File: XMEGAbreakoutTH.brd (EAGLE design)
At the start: 62.2 x 48.3 mm, 26 parts, among them IC1 XMEGA16A4

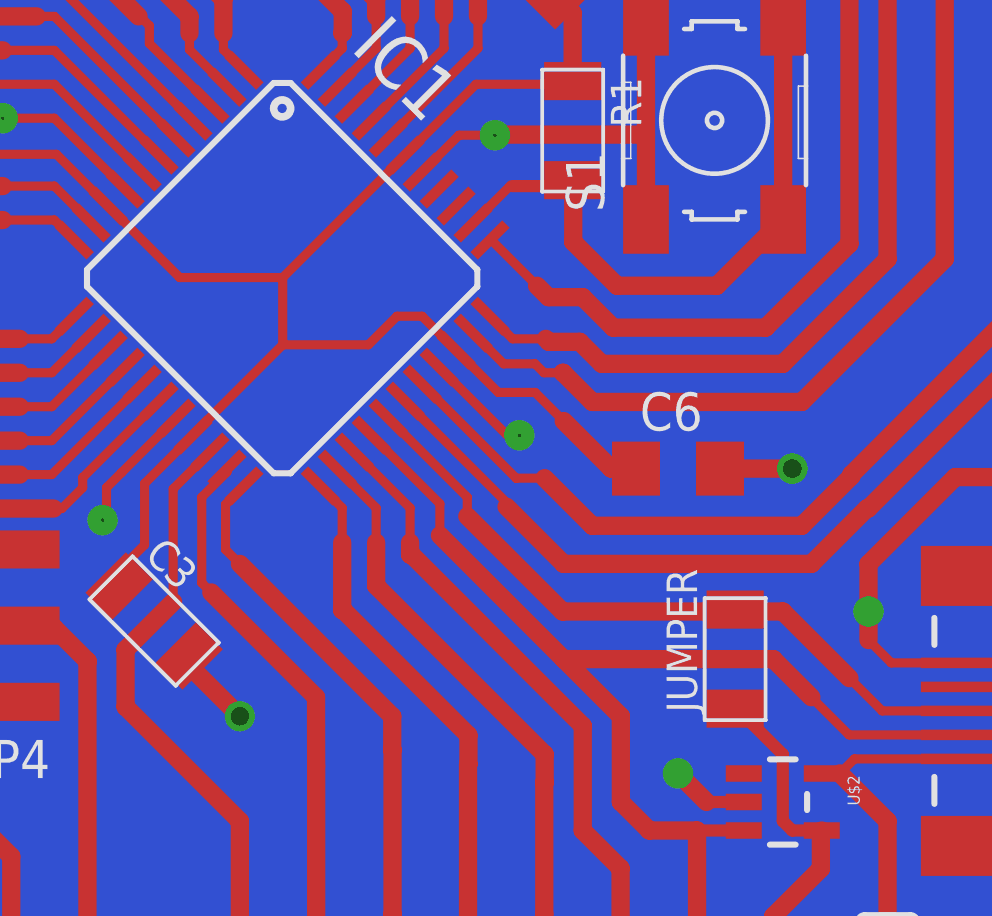
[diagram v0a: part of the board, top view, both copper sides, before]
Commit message: 600dpi
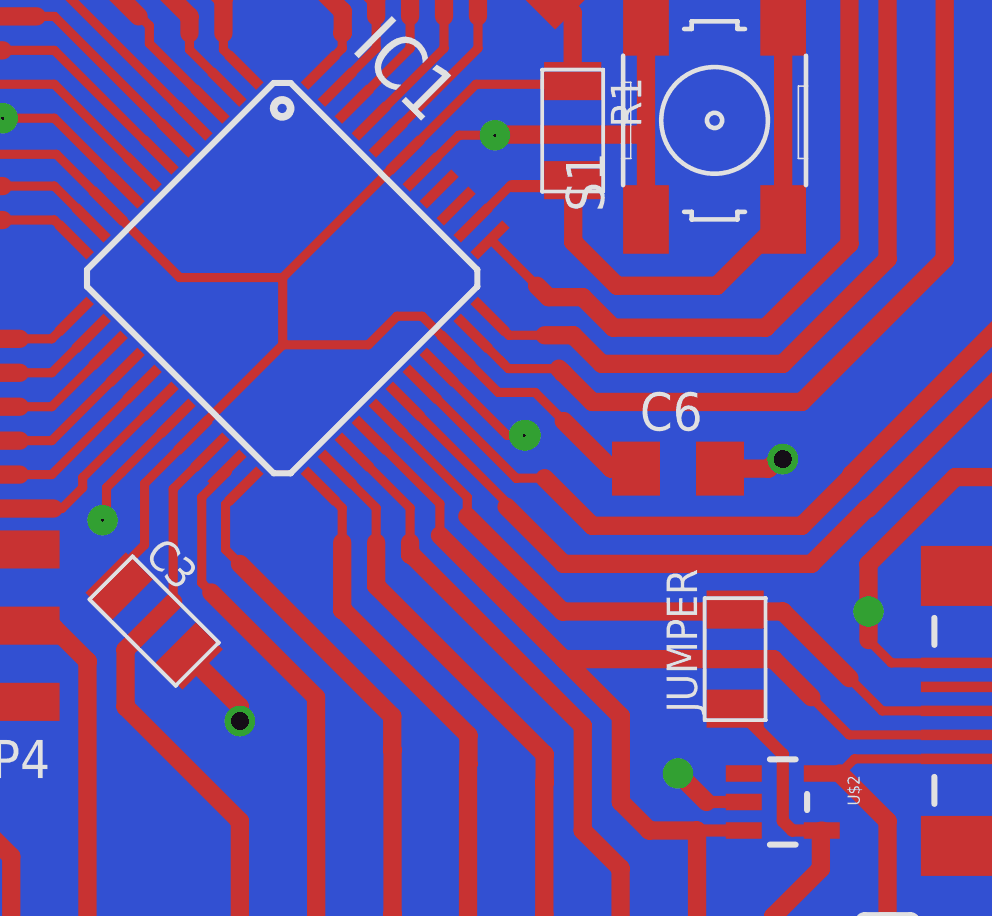
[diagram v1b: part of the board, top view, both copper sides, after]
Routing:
- net GND: track 239.0 -> 259.3 mm, vias 11 -> 14
